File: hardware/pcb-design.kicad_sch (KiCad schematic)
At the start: 133 parts, among them SW1 SW_MEC_5G, SW10 SW_MEC_5G, SW11 SW_MEC_5G, SW12 SW_MEC_5G, SW13 SW_MEC_5G, SW14 SW_MEC_5G, SW15 SW_MEC_5G, SW16 SW_MEC_5G, SW17 SW_MEC_5G, SW18 SW_MEC_5G, SW19 SW_MEC_5G, SW2 SW_MEC_5G, SW20 SW_MEC_5G, SW21 SW_MEC_5G, SW22 SW_MEC_5G, SW23 SW_MEC_5G, SW24 SW_MEC_5G, SW25 SW_MEC_5G, SW26 SW_MEC_5G, SW27 SW_MEC_5G, SW28 SW_MEC_5G, SW29 SW_MEC_5G, SW3 SW_MEC_5G, SW30 SW_MEC_5G, SW31 SW_MEC_5G, SW32 SW_MEC_5G, SW33 SW_MEC_5G, SW34 SW_MEC_5G, SW35 SW_MEC_5G, SW36 SW_MEC_5G, SW37 SW_MEC_5G, SW38 SW_MEC_5G, SW39 SW_MEC_5G, SW4 SW_MEC_5G, SW40 SW_MEC_5G, SW41 SW_MEC_5G, SW42 SW_MEC_5G, SW43 SW_MEC_5G, SW44 SW_MEC_5G, SW45 SW_MEC_5G, SW46 SW_MEC_5G, SW47 SW_MEC_5G, SW48 SW_MEC_5G, SW49 SW_MEC_5G, SW5 SW_MEC_5G, SW50 SW_MEC_5G, SW51 SW_MEC_5G, SW52 SW_MEC_5G, SW53 SW_MEC_5G, SW54 SW_MEC_5G, SW55 SW_MEC_5G, SW56 SW_MEC_5G, SW57 SW_MEC_5G, SW58 SW_MEC_5G, SW59 SW_MEC_5G, SW6 SW_MEC_5G, SW60 SW_MEC_5G, SW61 SW_MEC_5G, SW62 SW_MEC_5G, SW63 SW_MEC_5G, SW64 SW_MEC_5G, SW65 SW_MEC_5G, SW66 SW_MEC_5G, SW7 SW_MEC_5G, SW8 SW_MEC_5G, SW9 SW_MEC_5G

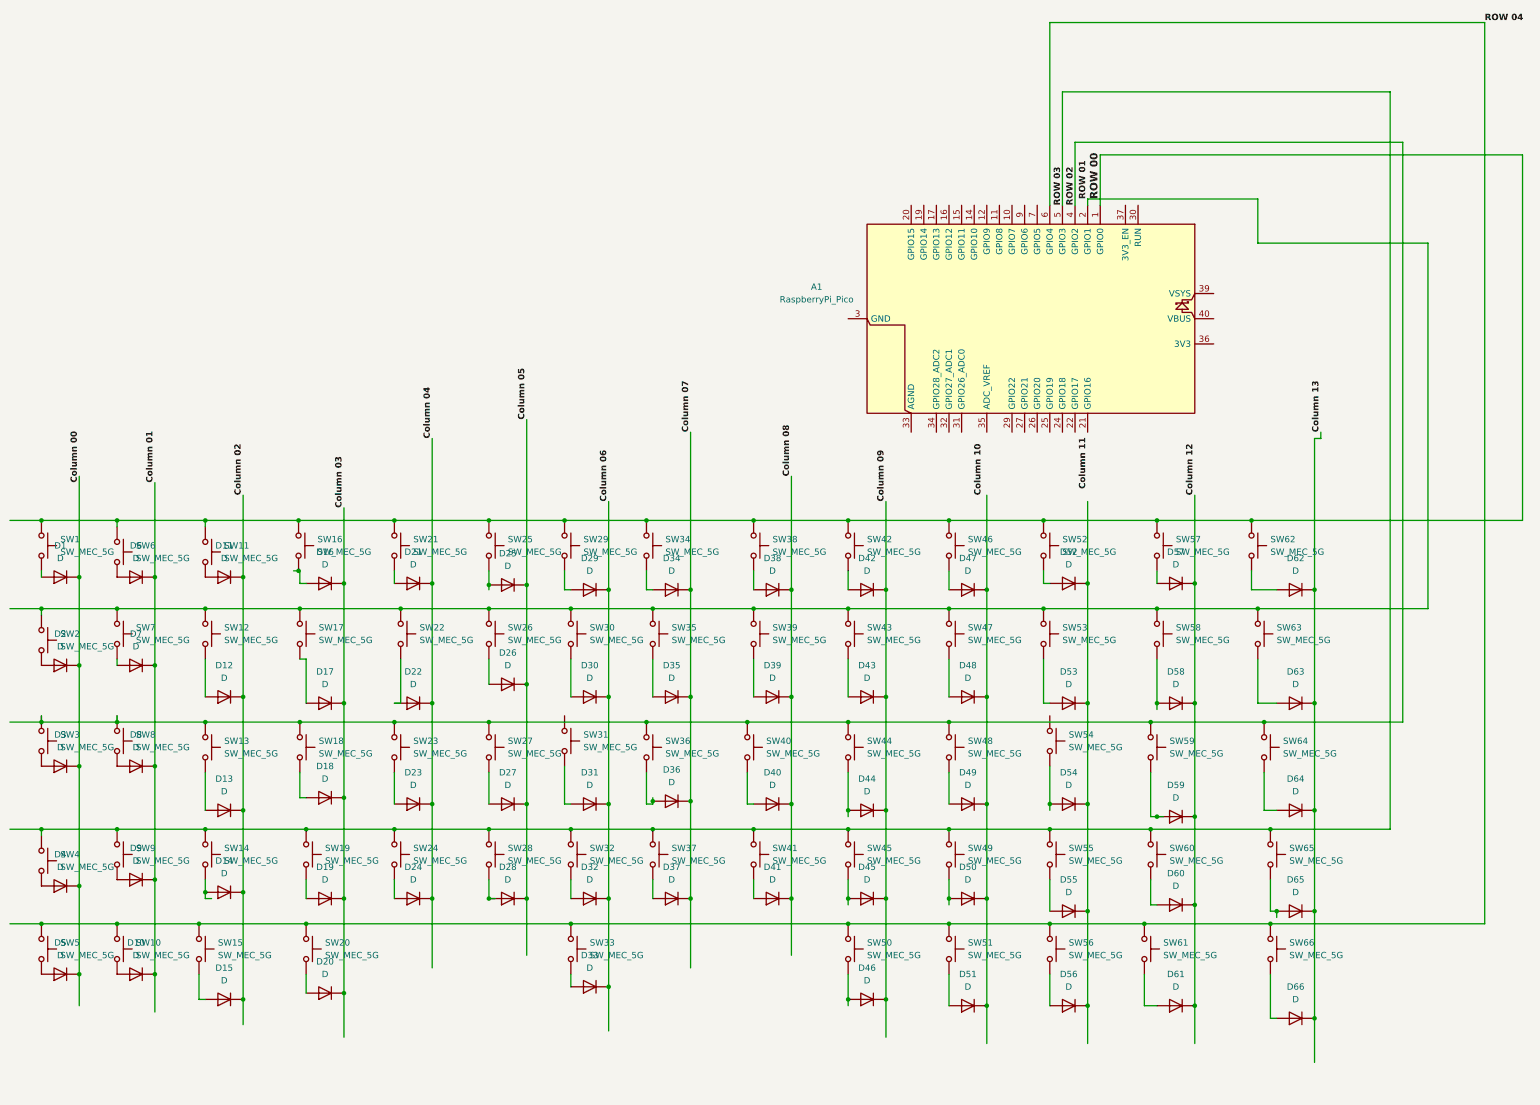
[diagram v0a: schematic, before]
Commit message: Schemantic done
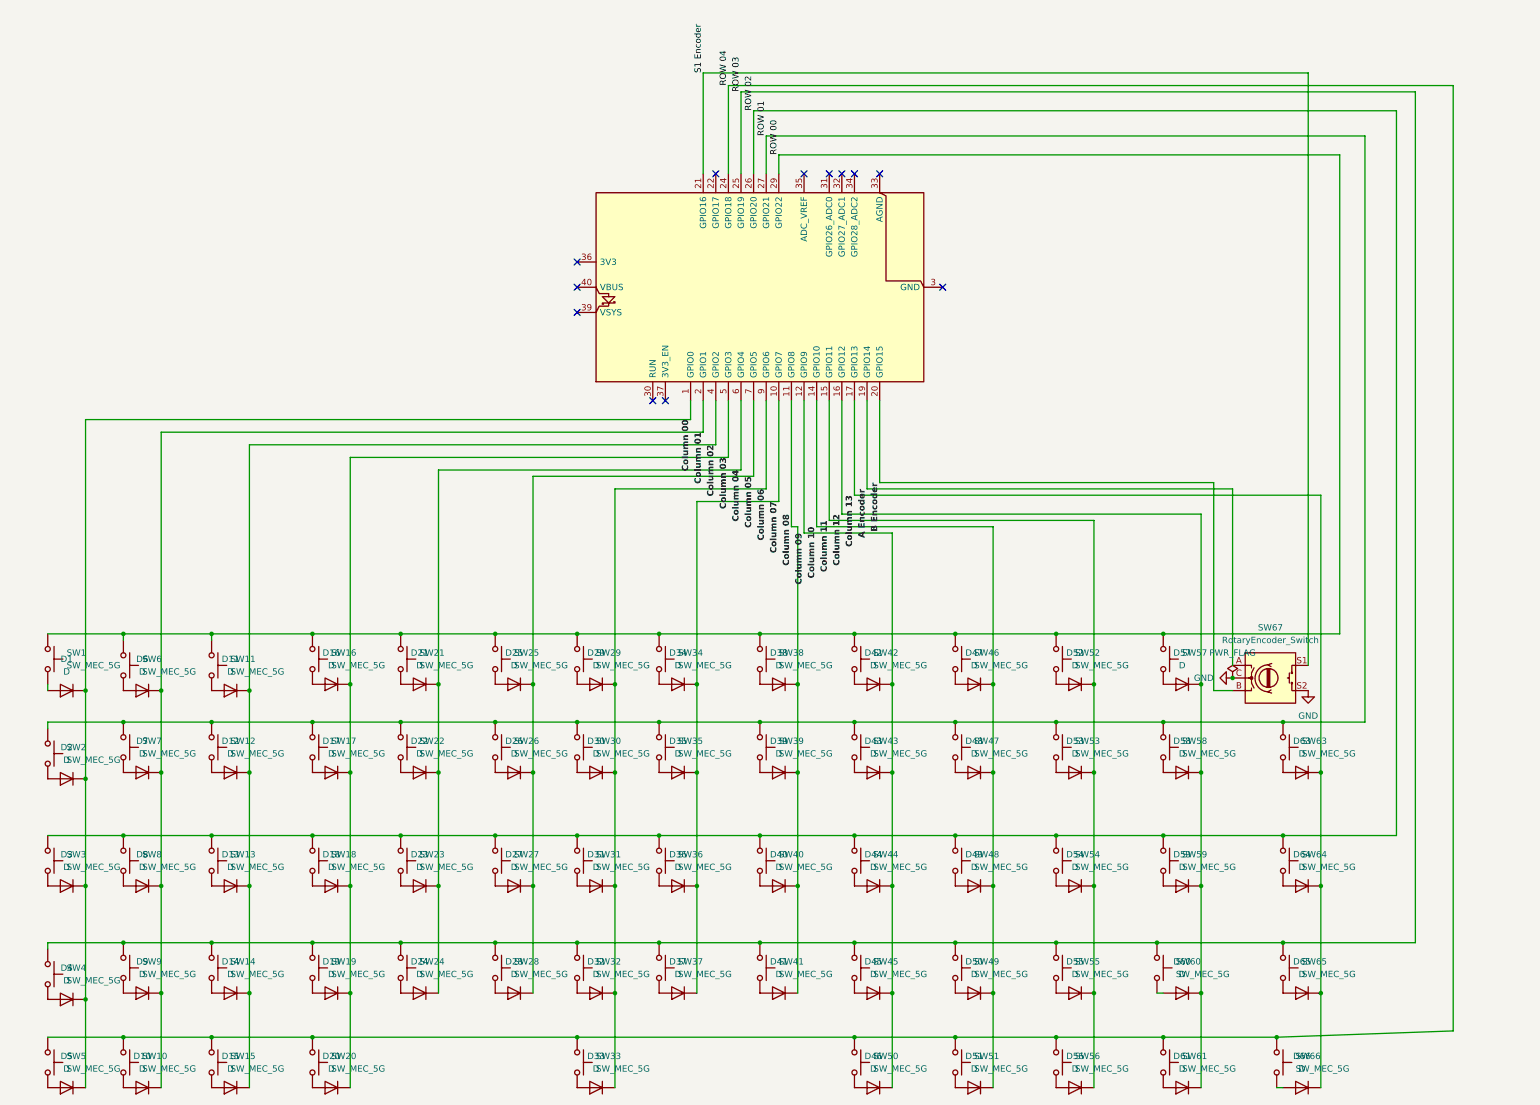
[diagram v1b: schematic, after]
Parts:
- removed D62: D, symbol Device:D
- removed SW62: SW_MEC_5G, symbol Switch:SW_MEC_5G
- added SW67: RotaryEncoder_Switch, symbol Device:RotaryEncoder_Switch
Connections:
- net Column 00: now also A1.1 (GPIO0)
- net Column 01: now also A1.2 (GPIO1)
- net Column 02: now also A1.4 (GPIO2)
- net Column 03: now also A1.5 (GPIO3)
- net Column 04: now also A1.6 (GPIO4)
- net Column 05: now also A1.7 (GPIO5)
- net Column 06: now also A1.9 (GPIO6)
- net Column 07: now also A1.10 (GPIO7)
- net Column 08: now also A1.11 (GPIO8)
- net Column 09: now also A1.12 (GPIO9)
- net Column 10: now also A1.14 (GPIO10), D47.1 (K), D48.1 (K), D49.1 (K), D50.1 (K), D51.1 (K)
- net Column 11: now also A1.15 (GPIO11), D52.1 (K), D53.1 (K), D54.1 (K), D55.1 (K), D56.1 (K)
- net Column 12: now also A1.16 (GPIO12)
- net Column 13: now also A1.17 (GPIO13)
- net ROW 00: now also A1.29 (GPIO22); no longer A1.1 (GPIO0), A1.2 (GPIO1), SW12.1 (A), SW12.2 (A), SW17.1 (A), SW17.2 (A), SW2.1 (A), SW2.2 (A), SW22.1 (A), SW22.2 (A), SW26.1 (A), SW26.2 (A), SW30.1 (A), SW30.2 (A), SW35.1 (A), SW35.2 (A), SW39.1 (A), SW39.2 (A), SW43.1 (A), SW43.2 (A), SW47.1 (A), SW47.2 (A), SW53.1 (A), SW53.2 (A), SW58.1 (A), SW58.2 (A), SW63.1 (A), SW63.2 (A), SW7.1 (A), SW7.2 (A)
- net ROW 02: now also A1.26 (GPIO20), SW31.1 (A), SW31.2 (A), SW54.1 (A), SW54.2 (A); no longer A1.4 (GPIO2)
- net ROW 03: now also A1.25 (GPIO19); no longer A1.5 (GPIO3)
- net ROW 04: now also A1.24 (GPIO18); no longer A1.6 (GPIO4)
- net A Encoder: now reaches A1.19 (GPIO14)
- net A Encoder: now also SW67.A
- net B Encoder: now reaches A1.20 (GPIO15)
- net B Encoder: now also SW67.B
- net S1 Encoder: now reaches A1.21 (GPIO16)
- net S1 Encoder: now also SW67.S1
- net ROW 01: now reaches A1.27 (GPIO21)
- net ROW 01: now also SW12.1 (A), SW12.2 (A), SW17.1 (A), SW17.2 (A), SW2.1 (A), SW2.2 (A), SW22.1 (A), SW22.2 (A), SW26.1 (A), SW26.2 (A), SW30.1 (A), SW30.2 (A), SW35.1 (A), SW35.2 (A), SW39.1 (A), SW39.2 (A), SW43.1 (A), SW43.2 (A), SW47.1 (A), SW47.2 (A), SW53.1 (A), SW53.2 (A), SW58.1 (A), SW58.2 (A), SW63.1 (A), SW63.2 (A), SW7.1 (A), SW7.2 (A)
- new net GND: SW67.C, SW67.S2
- no-connect marks 0 -> 12
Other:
- moved on the sheet: D1, D10, D11, D12, D13, D14, D15, D16, D17, D18, D19, D2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
